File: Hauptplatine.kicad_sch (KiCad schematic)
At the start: 16 parts, among them J7 Conn_01x12_Female, M1 Conn_01x10_Female, M2 Conn_01x10_Female, M3 Conn_01x10_Female, M4 Conn_01x10_Female, M5 Conn_01x10_Female, U2 esp32_dev4_left, U3 esp32_dev4_right

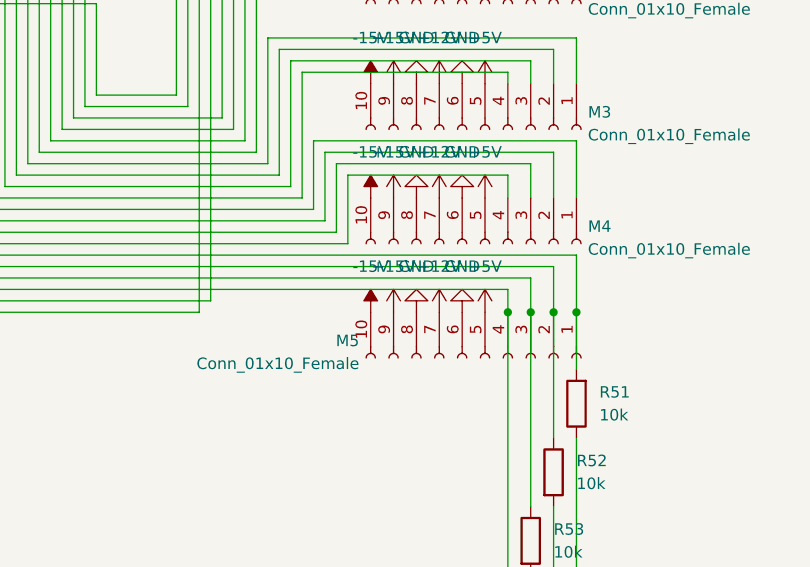
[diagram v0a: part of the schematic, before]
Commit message: final Design V2
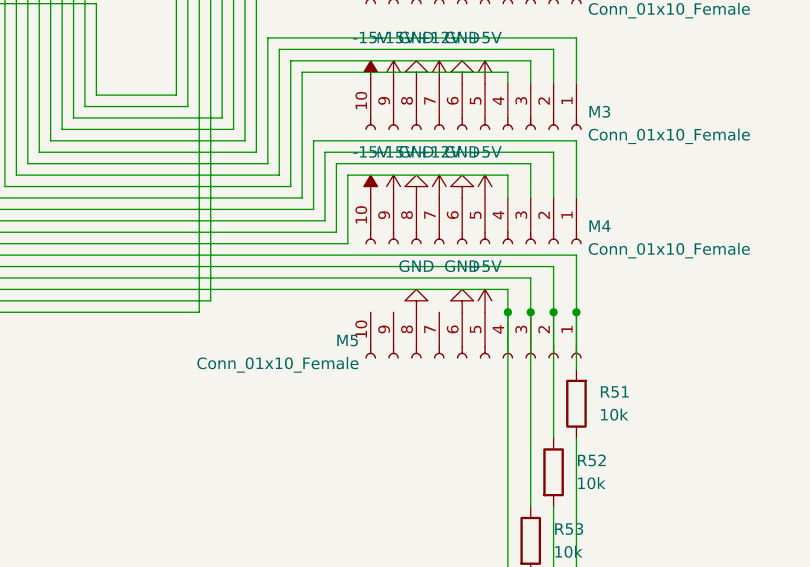
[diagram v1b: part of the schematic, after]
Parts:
- R51, R52, R53, R54: footprint Resistor_THT:R_Axial_DIN0411_L9.9mm_D3.6mm_P12.70mm_Horizontal -> Resistor_SMD:R_0805_2012Metric_Pad1.20x1.40mm_HandSolder
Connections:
- net +12V: no longer M5.7 (Pin_7)
- net +15V: no longer M5.9 (Pin_9)
- net -15V: no longer M5.10 (Pin_10)
